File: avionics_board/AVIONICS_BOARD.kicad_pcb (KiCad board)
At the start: 4 copper layers, 80 x 80 mm, 161 parts, among them J1 Conn_02x03_Odd_Even, J10 Conn_02x03_Odd_Even, J11 Conn_02x03_Odd_Even, J12 Conn_02x03_Odd_Even, J13 Conn_02x03_Odd_Even, J14 Conn_02x05_Odd_Even, J15 Conn_02x05_Odd_Even, J2 Conn_02x03_Odd_Even, J3 Conn_02x03_Odd_Even, J4 Conn_02x03_Odd_Even, J5 Conn_01x06, J6 Conn_01x04, J7 PC104 Conn_02x20_Odd_Even, J8 Conn_02x04, J9 10155435-00011LF, SW1 EVP-AA602W, SW2 SW_DIP_x01, SW3 EVP-AA602W, U1 STM32L496ZGTx, U10 TCAN3414, U11 TCAN3414, U12 74LVC2G07, U13 INA226, U14 DRV8838, U15 TCA9548APWR, U16 AP3602AKTR-G1, U2 MMC5983MA, U3 BMI270, U4 INA226, U5 DRV8838, U6 TPL5010, U7 INA226, U8 DRV8838, U9 MR25H10, X1 10MHz, X2 32.768KHZ

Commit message: propate the changes to RF
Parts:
- R6: value 300K -> 330K
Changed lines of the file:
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@@
 			)
 		)
-		(property "Value" "300K"
+		(property "Value" "330K"
 			(at 0 1.17 45)
 			(layer "F.Fab")
@@
 			)
 		)
-		(property "Part Number" "RC0402FR-07300KL"
+		(property "Part Number" "RC0402FR-07330KL"
 			(at 0 0 45)
 			(unlocked yes)

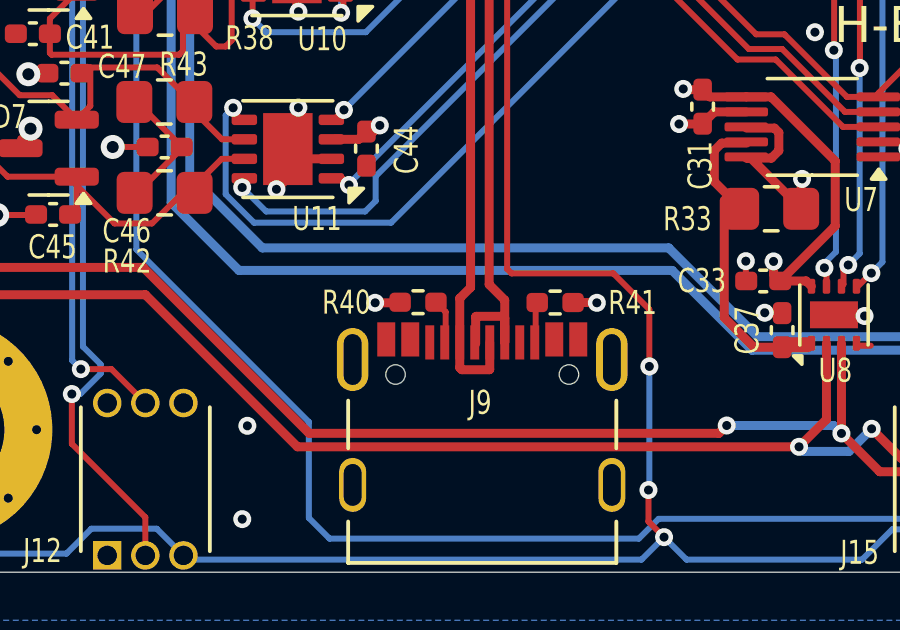
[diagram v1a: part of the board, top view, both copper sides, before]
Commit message: tweaks before merge
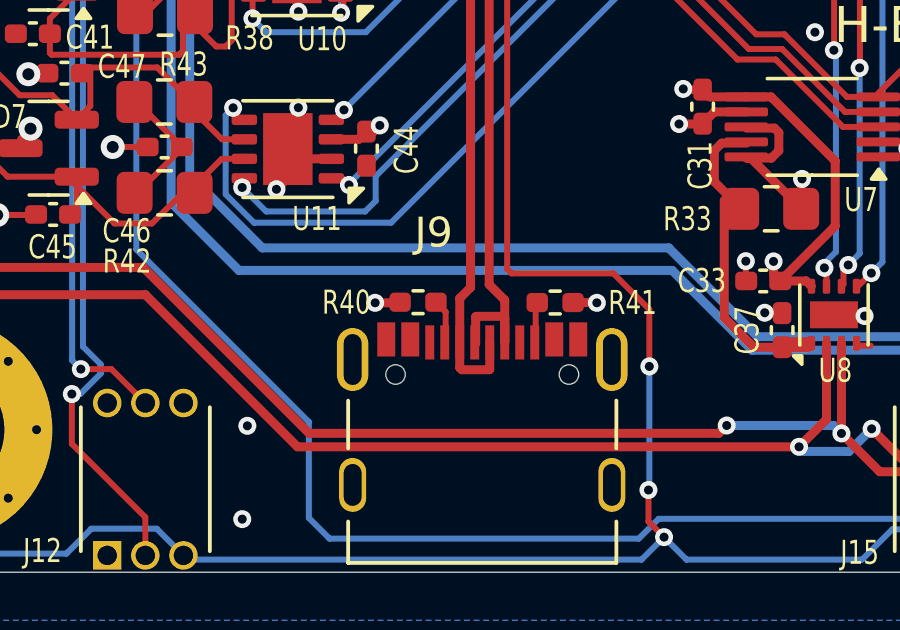
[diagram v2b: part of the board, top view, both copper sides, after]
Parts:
- J9: footprint Project:AMPHENOL_10155435-00011LF -> Common:AMPHENOL_10155435-00011LF
